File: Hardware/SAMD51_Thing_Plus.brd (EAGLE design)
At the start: 33 x 58.9 mm, 53 parts, among them J4 CORTEX_DEBUG_PTH, J5 455-1750-1-ND, J6 AMP FCI 10103594-0001LF, Q1 2.5A/30V, U1 MCP73831, U2 ATSAMD51J20A-A, U3 AP2112K-3.3V, U4 RFM69HW, Y1 32.768kHz

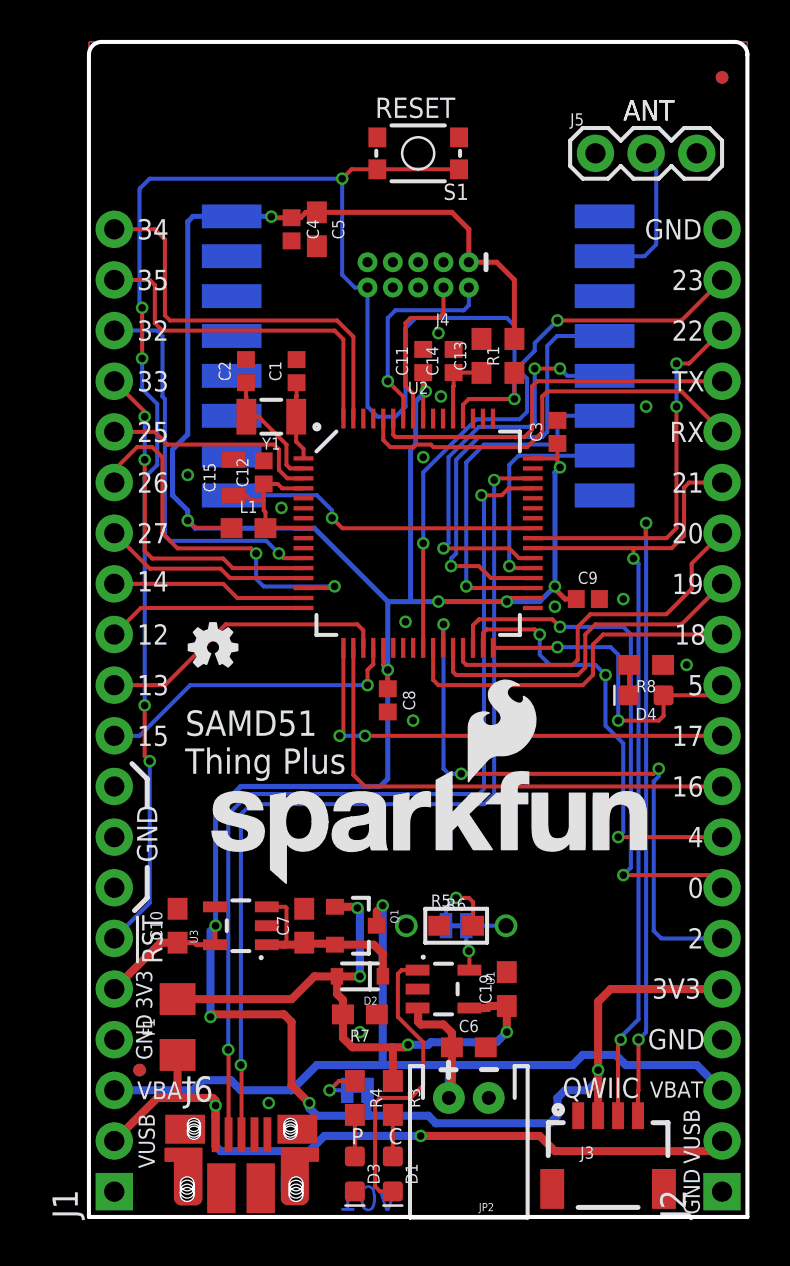
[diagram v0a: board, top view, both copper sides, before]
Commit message: Buzzard Text
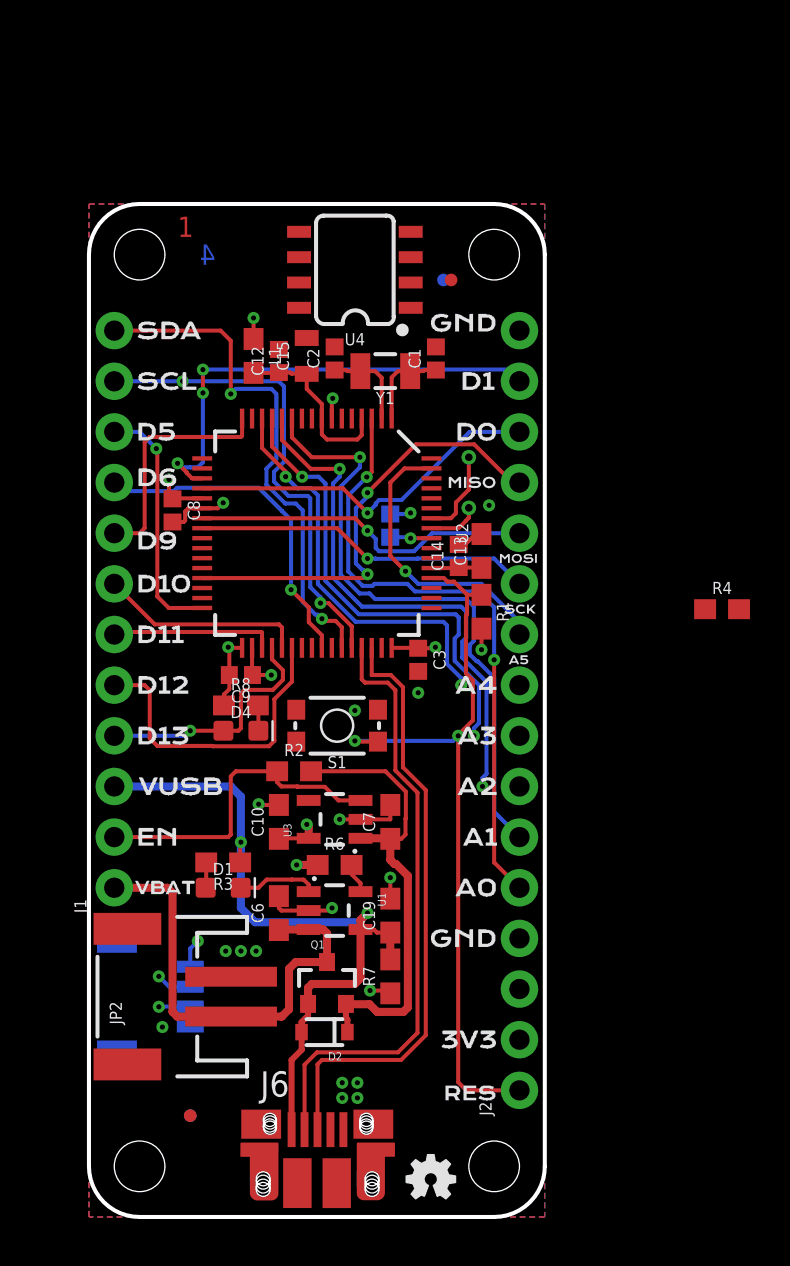
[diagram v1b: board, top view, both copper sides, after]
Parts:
- removed C4: 0.1uF, SparkFun-Capacitors:0402
- removed C5: 10uF, SparkFun-Capacitors:0603
- removed D3: RED, SparkFun-LED:LED-0603
- removed F1: 6V/0.75A, SparkFun-Fuses:1206
- removed J4: CORTEX_DEBUG_PTH, SparkFun-Connectors:2X5-PTH-1.27MM
- removed J5: 455-1750-1-ND, SparkFun-Connectors:1X03
- removed LOGO1: SFE_LOGO_NAME_FLAME.2_INCH, SparkFun-Aesthetics:SFE_LOGO_NAME_FLAME_.2
- removed LOGO3: SFE_LOGO_NAME.2_INCH, SparkFun-Aesthetics:SFE_LOGO_NAME_.2
- removed R5: DNP, SparkFun-Passives:1/6W-RES
- removed SJ1, SJ2: JUMPER-PAD-2-NC_BY_TRACE, SparkFun-Passives:PAD-JUMPER-2-NC_BY_TRACE_YES_SILK
- added R2: 10k, SparkFun-Resistors:0603
- added TP1, TP2: TEST-POINTTP_15TH_THRU, SparkFun-Connectors:TP_15TH
- added U$10: (no value), buzzard_labels (1):A518
- added U$11: (no value), buzzard_labels (1):A419
- added U$12: (no value), buzzard_labels (1):D014
- added U$13: (no value), buzzard_labels (1):D52
- added U$14: (no value), buzzard_labels (1):D63
- added U$15: (no value), buzzard_labels (1):D94
- added U$16: (no value), buzzard_labels (1):D105
- added U$17: (no value), buzzard_labels (1):D113
- added U$18: (no value), buzzard_labels (1):D116
- added U$19: (no value), buzzard_labels (1):D139
- added U$20: (no value), buzzard_labels (1):D1210
- added U$21: (no value), buzzard_labels (1):EN7
- added U$22, U$23: (no value), buzzard_labels (1):GND12
- added U$24: (no value), buzzard_labels (2):VBAT25
- added U$25: (no value), buzzard_labels (1):MOSI16
- added U$26: (no value), buzzard_labels (1):SCK17
- added U$27: (no value), buzzard_labels (1):SCL1
- added U$28: (no value), buzzard_labels (1):SDA0
- added U$29: (no value), buzzard_labels (2):MISO26
- added U$30: (no value), buzzard_labels (1):VUSB11
- added U$31: (no value), buzzard_labels (3):#RES21
- added U$32: (no value), buzzard_labels (3):A524
- added U$33: (no value), buzzard_labels (3):3V320
- added U$34: (no value), buzzard_labels (3):A018
- added U$35: (no value), buzzard_labels (3):A117
- added U$36: (no value), buzzard_labels (3):A216
- added U$37: (no value), buzzard_labels (3):A315
- added U$38: (no value), buzzard_labels (3):A414
- added U$39: (no value), buzzard_labels (3):GND11
- added U$4: (no value), buzzard_labels (1):#RES26
- added U$40: (no value), buzzard_labels (3):SCK25
- added U$41: (no value), buzzard_labels (3):MOSI26
- added U$42: (no value), buzzard_labels (3):MISO23
- added U$43: (no value), buzzard_labels (3):D013
- added U$44: (no value), buzzard_labels (3):D105
- added U$45: (no value), buzzard_labels (3):D112
- added U$46: (no value), buzzard_labels (3):D116
- added U$47: (no value), buzzard_labels (3):D129
- added U$48: (no value), buzzard_labels (3):D138
- added U$49: (no value), buzzard_labels (3):VUSB10
- added U$5: (no value), buzzard_labels (1):3V325
- added U$50: (no value), buzzard_labels (3):EN7
- added U$51: (no value), buzzard_labels (3):VBAT22
- added U$52: (no value), buzzard_labels (3):D94
- added U$53: (no value), buzzard_labels (3):D63
- added U$54: (no value), buzzard_labels (3):D52
- added U$55: (no value), buzzard_labels (3):SCL1
- added U$56: (no value), buzzard_labels (3):SDA0
- added U$57: (no value), buzzard_labels (3):GND19
- added U$6: (no value), buzzard_labels (1):A023
- added U$7: (no value), buzzard_labels (1):A122
- added U$8: (no value), buzzard_labels (1):A221
- added U$9: (no value), buzzard_labels (1):A320
- J1: device SparkFun-Connectors:1X20_NOSILK -> SparkFun-Connectors:1X12_NO_SILK
- J2: device SparkFun-Connectors:1X20_NOSILK -> SparkFun-Connectors:1X16_NO_SILK
- JP2: device SparkFun-Connectors:JST-2-PTH -> SparkFun-Connectors:JST-2-SMD
- R4: value 1K -> 10k
- S1: device SparkFun-Electromechanical:TACTILE_SWITCH_SMD_4.6X2.8MM -> SparkFun-Switches:TACTILE_SWITCH_SMD_4.6X2.8MM
- U4: value RFM69HW -> 4MB Flash; device SparkFun-RF:RFM69W-XXXS2 -> SparkFun-IC-Memory:SO08
- moved R4 30.7 mm to (31.8, 30.5), turned to 0 degrees
- moved S1 29.0 mm to (12.4, 24.6)
- moved LOGO2 28.8 mm to (17.1, 1.91)
- moved J3 21.8 mm to (5.08, 11.0), flipped to the bottom, turned to 90 degrees
- moved R8 20.4 mm to (7.62, 25.7), turned to 0 degrees
- moved D4 20.4 mm to (7.62, 24.4), turned to 270 degrees
- moved C9 17.8 mm to (7.62, 27.2), turned to 180 degrees
- moved FD4 17.3 mm to (17.8, 47.0)
- moved FD2 17.0 mm to (18.2, 47.0)
- moved D1 16.7 mm to (6.73, 16.5), turned to 270 degrees
- moved JP2 16.4 mm to (3.43, 11.0), turned to 90 degrees
- moved J1 15.2 mm to (1.27, 16.5)
- moved R3 14.6 mm to (6.73, 17.8), turned to 180 degrees
- moved C8 14.4 mm to (4.19, 35.4)
- moved C3 13.4 mm to (16.5, 27.9), turned to 270 degrees
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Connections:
- removed net 0: J2.7, U2.30
- removed net 12: J1.12, U2.16
- removed net 13: J1.11, U2.19
- removed net 14: J1.13, U2.15
- removed net 15: J1.10, U2.20
- removed net 16: J2.9, U2.18
- removed net 17: J2.10, U2.17
- removed net 18: J2.12, U2.26
- removed net 19: J2.13, U2.28
- removed net 2: J2.6, U2.27
- removed net 20: J2.14, U2.29
- removed net 21: J2.15, J3.3, U2.39
- removed net 22: J2.18, J3.4, U2.40
- removed net 23: J2.19, U2.25
- removed net 25: J1.16, U2.3
- removed net 26: J1.15, U2.14
- removed net 27: J1.14, U2.13
- removed net 32: J1.18, U2.11
- removed net 33: J1.17, U2.12
- removed net 34: J1.20, U2.63
- removed net 35: J1.19, U2.64
- removed net 4: J2.8, U2.31
- removed net 5: D4.A, J2.11, U2.32
- removed net N$16: R6.2, SJ1.1
- removed net N$2: D3.A, R4.2
- removed net N$3: R4.1, SJ2.1
- removed net N$4: J5.2, U4.10
- removed net RFM_MISO: U2.38, U4.13
- removed net RFM_MOSI: U2.35, U4.14
- removed net RFM_RESET: U2.41, U4.1
- removed net RFM_SCK: U2.36, U4.12
- removed net RFM_SS: U2.37, U4.15
- removed net U0RXD: J2.16, U2.60
- removed net U0TXD: J2.17, U2.59
- removed net VUSB-RAW: F1.1, J1.2, J2.2, J6.VBUS
- new net A0: J2.5, U2.3
- new net A1: J2.6, U2.11
- new net A2: J2.7, U2.12
- new net A3: J2.8, U2.13
- new net A4: J2.9, U2.14
- new net A5: J2.10, U2.63
- new net D0: J2.14, U2.20
- new net D1: J2.15, U2.19
- new net D10: J1.7, U2.37
- new net D11: J1.6, U2.35
- new net D12: J1.5, U2.38
- new net D13: D4.A, J1.4, U2.36
- new net D2_FLASH_MISO: U2.31
- new net D3_FLASH_SCK: U2.18
- new net D4_FLASH_MOSI: U2.17
- new net D5: J1.10, U2.32
- new net D6: J1.9, U2.41
- new net D7: U2.42
- new net D8: U2.15
- new net D9: J1.8, U2.16
- new net EN: J1.2, R2.1, U3.3
- new net FLASH_CS: R4.1, U2.30, U4.1
- new net MISO: J2.13, U2.29
- new net MOSI: J2.12, U2.23
- new net RXD: U2.50
- new net RXLED: U2.64
- new net SCK: J2.11, U2.24
- new net SCL: J1.11, J3.4, U2.44
- new net SDA: J1.12, J3.3, U2.43
- new net TXD: U2.49
- new net TXLED: U2.51
- net !RESET: now also J2.1; no longer J1.6, J4.10, S1.3
- net 3.3V: now also J2.2, R4.2; no longer C4.1, C5.1, J1.5, J2.5, J4.1, SJ2.2
- net GND: now also J2.16, JP2.2; no longer C4.2, C5.2, D3.C, J1.1, J1.4, J1.7, J1.8, J1.9, J2.1, J2.20, J4.3, J4.5, J5.1, J5.3, JP2.1, R5.1, S1.2, U4.11, U4.9
- net N$14: now also R6.2; no longer R5.2, SJ1.2
- net SWDCLK: now also TP2.P$1; no longer J4.4
- net SWDIO: now also TP1.P$1; no longer J4.2
- net VIN: now also R2.2; no longer U3.3
- net V_BATT: now also J1.1, JP2.1; no longer J1.3, J2.3, JP2.2
- net V_USB: now also J1.3, J6.VBUS; no longer F1.2
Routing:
- net 3.3V: track 162.1 -> 15.1 mm, vias 12 -> 8
- net SDA: track 0.00 -> 62.0 mm, vias 0 -> 3
- net SCL: track 0.00 -> 54.4 mm, vias 0 -> 3
- net !RESET: track 88.3 -> 37.5 mm, vias 6 -> 2
- net 22: track 49.3 -> 0.00 mm, vias 4 -> 0
- net 21: track 41.3 -> 0.00 mm, vias 2 -> 0
- net VUSB-RAW: track 38.3 -> 0.00 mm, vias 2 -> 0
- net 2: track 31.3 -> 0.00 mm, vias 3 -> 0
- net A1: track 0.00 -> 31.1 mm, vias 0 -> 1
- net A0: track 0.00 -> 30.9 mm, vias 0 -> 2
- net 23: track 29.8 -> 0.00 mm, vias 2 -> 0
- net A2: track 0.00 -> 28.8 mm, vias 0 -> 2
- net 0: track 26.9 -> 0.00 mm, vias 2 -> 0
- net V_BATT: track 49.2 -> 23.1 mm, vias 1 -> 0
- net A3: track 0.00 -> 26.1 mm, vias 0 -> 2
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- added copper zone on layer 15, net 3.3V
- added copper zone on layer 2, net GND
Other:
- board size 33 x 58.9 mm -> 22.9 x 50.8 mm
- board text added: "1"
- board text added: "3"
- board text removed: "!RST"
- board text removed: "0"
- board text removed: "12"
- board text removed: "13"
- board text removed: "14"
- board text removed: "15"
- board text removed: "16"
- board text removed: "17"
- board text removed: "18"
- board text removed: "19"
- board text removed: "20"
- board text removed: "21"
- board text removed: "22"
- board text removed: "23"
- board text removed: "25"
- board text removed: "26"
- board text removed: "27"
- board text removed: "32"
- board text removed: "33"
- board text removed: "34"
- board text removed: "35"
- board text removed: "3V3"
- board text removed: "5"
- board text removed: "ANT"
- board text removed: "C"
- board text removed: "CHG PROG"
- board text removed: "GND"
- board text removed: "P"
- board text removed: "PWR LED"
- board text removed: "QWIIC"
- board text removed: "RESET"
- board text removed: "RX"
- board text removed: "RXI"
- board text removed: "SAMD51 Thing Plus"
- board text removed: "TX"
- board text removed: "TXO"
- board text removed: "VBAT"
- board text removed: "VUSB"
- board text removed: "v01"
